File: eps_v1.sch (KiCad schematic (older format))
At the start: 5 parts

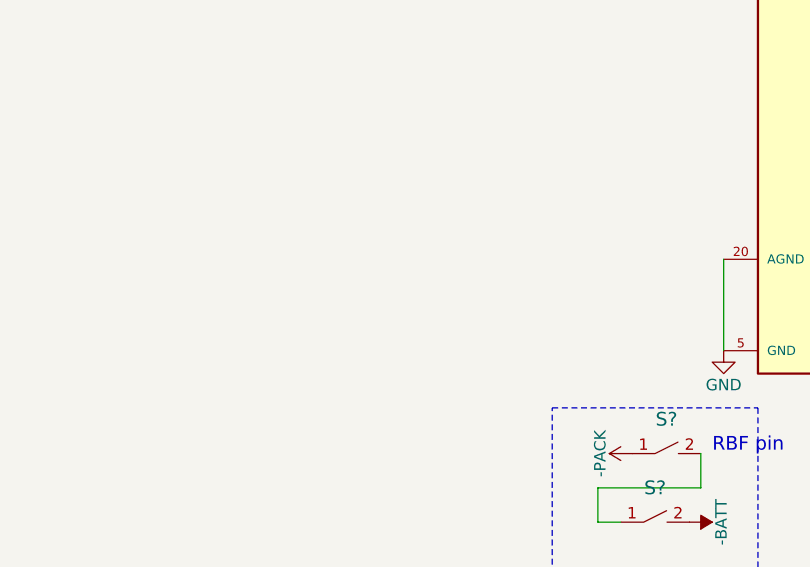
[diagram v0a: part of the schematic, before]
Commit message: Test commit
Wrote hello
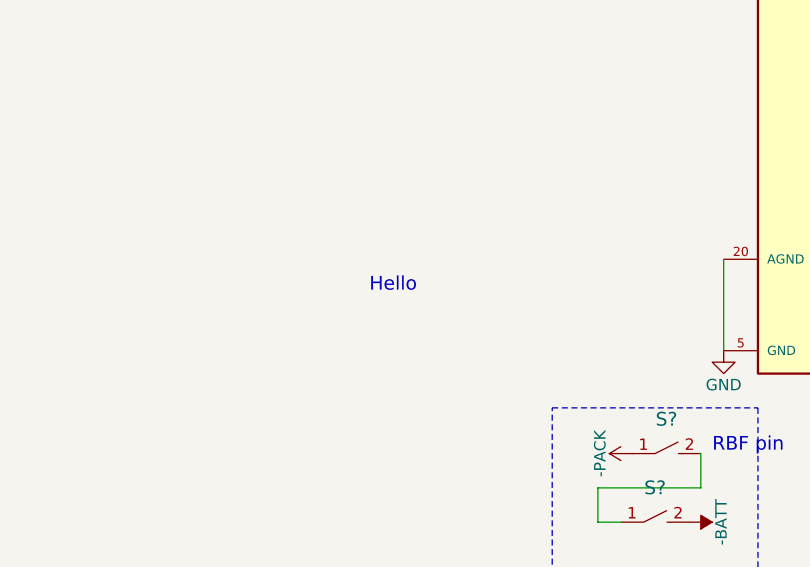
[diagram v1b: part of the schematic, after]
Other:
- note added: "Hello"
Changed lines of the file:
@@
 Text HLabel 2350 7200 0    60   Input ~ 0
 -YI
+Text Notes 3450 3950 0    60   ~ 0
+Hello
 $EndSCHEMATC
